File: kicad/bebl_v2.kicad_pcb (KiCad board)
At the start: 2 copper layers, 80 x 39 mm, 78 parts, among them P1 ISP, P10 LED_DRL, P11 DRV_LED, P12 CHG_LED, P13 LED_CHG, P2 FTDI, P3 LiPo, P4 USB-Micro, P5 Alt_Add, P6 Int1, P7 Int2, P8 DRL_LED, P9 LED_DRV, SW1 RST, SW2 MODE, U1 ATMEGA328, U2 FAN5346, U3 ADXL345, U4 MCP73831, U5 TPS61221DCK, X1 8MHz

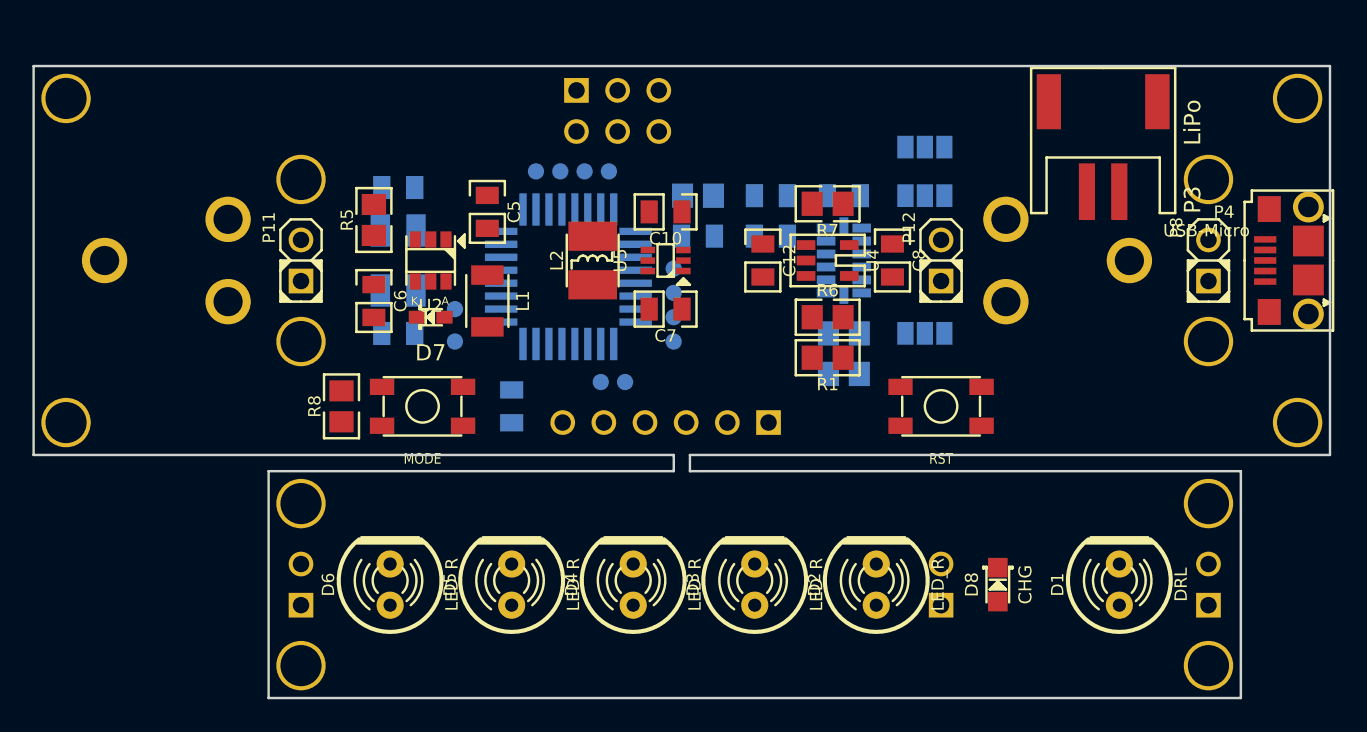
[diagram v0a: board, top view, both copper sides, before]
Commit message: bebl_v2 3d of housing, work in progress
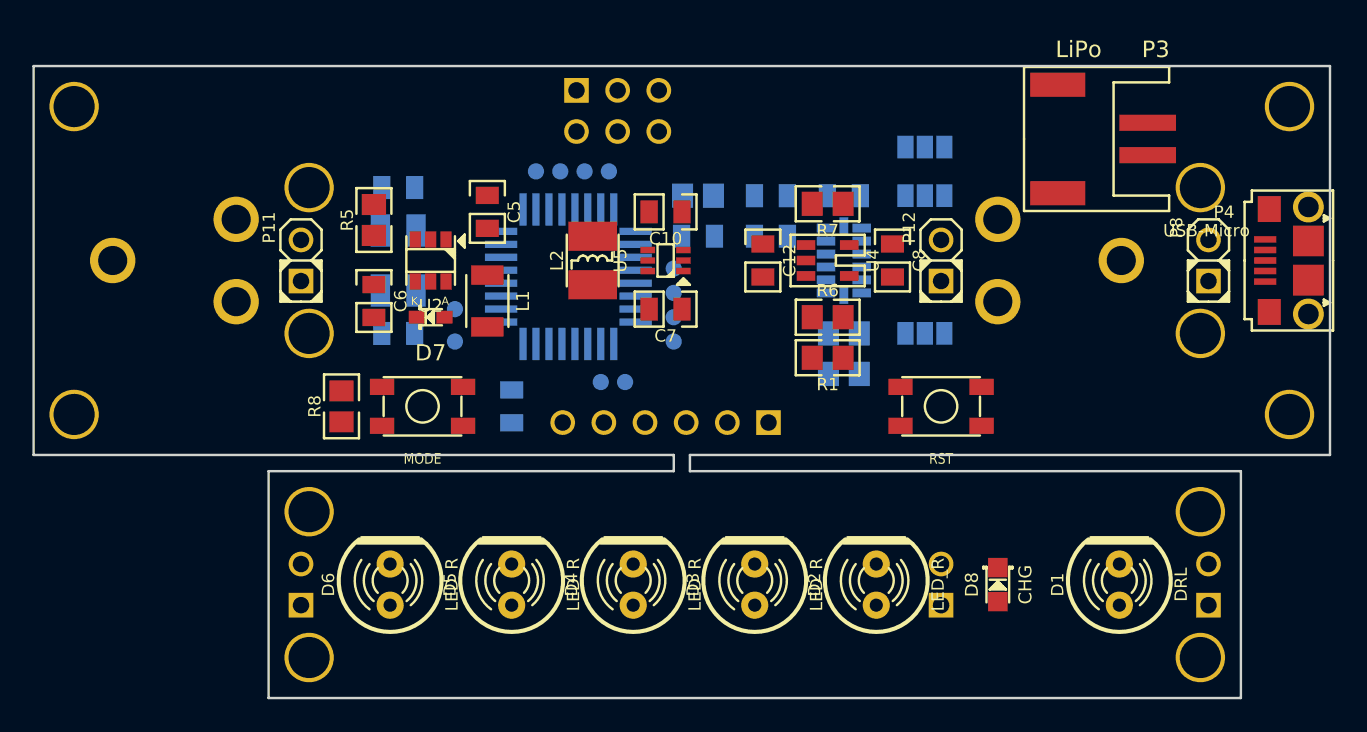
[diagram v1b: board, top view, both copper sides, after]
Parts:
- moved P3 6.02 mm to (99.5, 42.5), turned to 270 degrees
- moved SC1 0.71 mm to (40.5, 59.5)
- moved SC10 0.71 mm to (55.0, 74.5)
- moved SC11 0.71 mm to (110.0, 74.5)
- moved SC12 0.71 mm to (110.0, 65.5)
- moved SC2 0.71 mm to (115.5, 40.5)
- moved SC3 0.71 mm to (115.5, 59.5)
- moved SC4 0.71 mm to (40.5, 40.5)
- moved SC5 0.71 mm to (55.0, 54.5)
- moved SC6 0.71 mm to (55.0, 45.5)
- moved SC7 0.71 mm to (110.0, 45.5)
- moved SC8 0.71 mm to (110.0, 54.5)
- moved SC9 0.71 mm to (55.0, 65.5)
- moved B14 0.50 mm to (97.5, 50.0)
- moved B15 0.50 mm to (50.5, 50.0)
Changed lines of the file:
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@@
-(kicad_pcb (version 4) (host pcbnew "(2014-09-25 BZR 5147)-product")
+(kicad_pcb (version 4) (host pcbnew "(2014-jul-16 BZR unknown)-product")
   (general
     (links 143)
     (no_connects 143)
-    (area 37.8537 37.5442 118.521201 77.075001)
+    (area 36.399999 35.7817 119.600001 77.075001)
     (thickness 1.6)
-    (drawings 12)
+    (drawings 24)
     (tracks 0)
     (zones 0)
@@
   )
   (module bebl_v2_pretty:batt_clip (layer B.Cu)
-    (at 98 50 180)
+    (at 97.5 50 180)
     (fp_text reference B14 (at 3.556 0 450) (layer B.SilkS)
       (effects (font (size 1.5 1.5) (thickness 0.15)) (justify mirror))
@@
   )
   (module bebl_v2_pretty:batt_clip (layer B.Cu)
-    (at 50 50)
+    (at 50.5 50)
     (fp_text reference B15 (at 3.556 0 270) (layer B.SilkS)
       (effects (font (size 1.5 1.5) (thickness 0.15)) (justify mirror))
@@
   )
   (module bebl_v2_pretty:screw_3mm (layer F.Cu)
-    (at 110.5 65)
+    (at 110 65.5)
     (descr "vite 2,5mm")
     (fp_text reference SC12 (at 0 1.0795) (layer F.SilkS) hide
@@
   )
   (module bebl_v2_pretty:screw_3mm (layer F.Cu)
-    (at 110.5 75)
+    (at 110 74.5)
     (descr "vite 2,5mm")
     (fp_text reference SC11 (at 0 1.0795) (layer F.SilkS) hide
@@
   )
   (module bebl_v2_pretty:screw_3mm (layer F.Cu)
-    (at 54.5 75)
+    (at 55 74.5)
     (descr "vite 2,5mm")
     (fp_text reference SC10 (at 0 1.0795) (layer F.SilkS) hide
@@
   )
   (module bebl_v2_pretty:screw_3mm (layer F.Cu)
-    (at 54.5 65)
+    (at 55 65.5)
     (descr "vite 2,5mm")
     (fp_text reference SC9 (at 0 1.0795) (layer F.SilkS) hide
@@
   )
   (module bebl_v2_pretty:screw_3mm (layer F.Cu)
-    (at 110.5 55)
+    (at 110 54.5)
     (descr "vite 2,5mm")
     (fp_text reference SC8 (at 0 1.0795) (layer F.SilkS) hide
@@
   )
   (module bebl_v2_pretty:screw_3mm (layer F.Cu)
-    (at 110.5 45)
+    (at 110 45.5)
     (descr "vite 2,5mm")
     (fp_text reference SC7 (at 0 1.0795) (layer F.SilkS) hide
@@
   )
   (module bebl_v2_pretty:screw_3mm (layer F.Cu)
-    (at 54.5 45)
+    (at 55 45.5)
     (descr "vite 2,5mm")
     (fp_text reference SC6 (at 0 1.0795) (layer F.SilkS) hide
@@
   )
   (module bebl_v2_pretty:screw_3mm (layer F.Cu)
-    (at 54.5 55)
+    (at 55 54.5)
     (descr "vite 2,5mm")
     (fp_text reference SC5 (at 0 1.0795) (layer F.SilkS) hide
@@
   )
   (module bebl_v2_pretty:screw_3mm (layer F.Cu)
-    (at 40 60)
+    (at 40.5 59.5)
     (descr "vite 2,5mm")
     (fp_text reference SC1 (at 0 1.0795) (layer F.SilkS) hide
@@
   )
   (module bebl_v2_pretty:screw_3mm (layer F.Cu)
-    (at 116 40)
+    (at 115.5 40.5)
     (descr "vite 2,5mm")
     (fp_text reference SC2 (at 0 1.0795) (layer F.SilkS) hide
@@
   )
   (module bebl_v2_pretty:screw_3mm (layer F.Cu)
-    (at 116 60)
+    (at 115.5 59.5)
     (descr "vite 2,5mm")
     (fp_text reference SC3 (at 0 1.0795) (layer F.SilkS) hide
@@
   )
   (module bebl_v2_pretty:screw_3mm (layer F.Cu)
-    (at 40 40)
+    (at 40.5 40.5)
     (descr "vite 2,5mm")
     (fp_text reference SC4 (at 0 1.0795) (layer F.SilkS) hide
@@
   )
   (module bebl_v2_pretty:CONN_JST-2_SMD (layer F.Cu)
-    (at 104 38.5 180)
+    (at 99.5 42.5 270)
     (tags JST)
-    (fp_text reference P3 (at -5.5245 -7.747 450) (layer F.SilkS)
+    (fp_text reference P3 (at -5.5245 -7.747 540) (layer F.SilkS)
       (effects (font (size 1.016 1.016) (thickness 0.1524)))
     )
-    (fp_text value LiPo (at -5.5245 -2.9845 450) (layer F.SilkS)
+    (fp_text value LiPo (at -5.5245 -2.9845 540) (layer F.SilkS)
       (effects (font (size 1.016 1.016) (thickness 0.1524)))
     )
@@
     (fp_line (start 3.4925 -8.5725) (end 4.445 -8.5725) (layer F.SilkS) (width 0.1524))
     (fp_line (start 4.445 0.381) (end 0 0.381) (layer F.SilkS) (width 0.1524))
-    (pad "" smd rect (at -3.34772 -1.69926 180) (size 1.4986 3.39598) (layers F.Cu F.Paste F.Mask))
-    (pad 1 smd rect (at -0.99822 -7.24916 180) (size 0.99568 3.49758) (layers F.Cu F.Paste F.Mask)
+    (pad "" smd rect (at -3.34772 -1.69926 270) (size 1.4986 3.39598) (layers F.Cu F.Paste F.Mask))
+    (pad 1 smd rect (at -0.99822 -7.24916 270) (size 0.99568 3.49758) (layers F.Cu F.Paste F.Mask)
       (net 13 /BAT))
-    (pad 2 smd rect (at 0.99822 -7.24916 180) (size 0.99568 3.49758) (layers F.Cu F.Paste F.Mask)
-      (net 14 GND))
-    (pad "" smd rect (at 3.34772 -1.69926 180) (size 1.4986 3.39598) (layers F.Cu F.Paste F.Mask))
+    (pad 2 smd rect (at 0.99822 -7.24916 270) (size 0.99568 3.49758) (layers F.Cu F.Paste F.Mask)
+      (net 14 GND))
+    (pad "" smd rect (at 3.34772 -1.69926 270) (size 1.4986 3.39598) (layers F.Cu F.Paste F.Mask))
     (model /home/samata/projects-git/bebl_v2/kicad/3d_modules/s2b-ph-sm4-tb.wrl
       (at (xyz 0 0.254 0))
@@
     )
   )
+  (gr_line (start 38 43) (end 38 38) (angle 90) (layer Dwgs.User) (width 0.2))
+  (gr_line (start 43 43) (end 38 43) (angle 90) (layer Dwgs.User) (width 0.2))
+  (gr_line (start 43 38) (end 43 43) (angle 90) (layer Dwgs.User) (width 0.2))
+  (gr_line (start 38 38) (end 43 38) (angle 90) (layer Dwgs.User) (width 0.2))
+  (gr_line (start 118 38) (end 113 38) (angle 90) (layer Dwgs.User) (width 0.2))
+  (gr_line (start 118 43) (end 118 38) (angle 90) (layer Dwgs.User) (width 0.2))
+  (gr_line (start 113 43) (end 118 43) (angle 90) (layer Dwgs.User) (width 0.2))
+  (gr_line (start 113 38) (end 113 43) (angle 90) (layer Dwgs.User) (width 0.2))
+  (gr_line (start 119.5 63.5) (end 119.5 36.5) (angle 90) (layer Dwgs.User) (width 0.2))
+  (gr_line (start 36.5 63.5) (end 119.5 63.5) (angle 90) (layer Dwgs.User) (width 0.2))
+  (gr_line (start 36.5 36.5) (end 36.5 63.5) (angle 90) (layer Dwgs.User) (width 0.2))
+  (gr_line (start 119.5 36.5) (end 36.5 36.5) (angle 90) (layer Dwgs.User) (width 0.2))
   (gr_line (start 52.5 63) (end 77.5 63) (angle 90) (layer Edge.Cuts) (width 0.15))
   (gr_line (start 77.5 62) (end 38 62) (angle 90) (layer Edge.Cuts) (width 0.15))
